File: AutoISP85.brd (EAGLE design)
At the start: 10.5 x 38.1 mm, 4 parts, among them J1 MCU, J2 BOARD, U1 ATTINY85, U2 BOARD

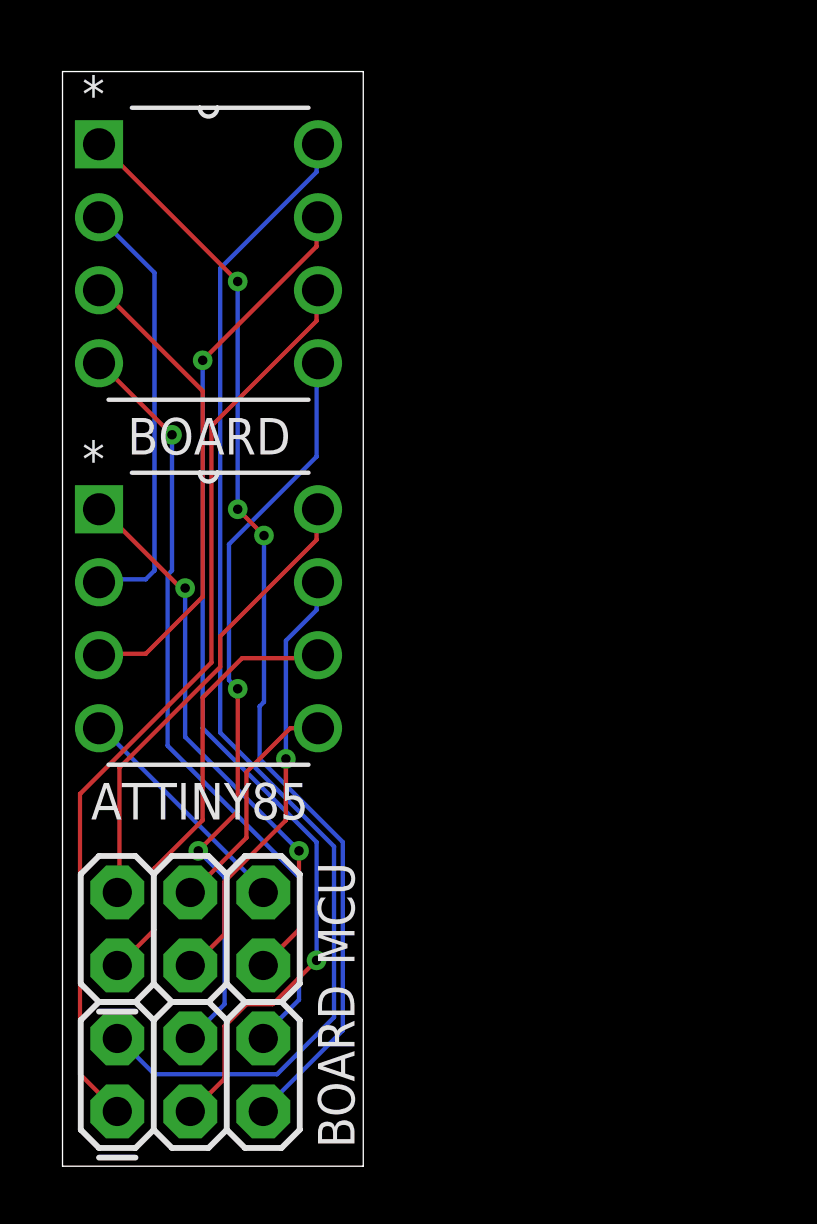
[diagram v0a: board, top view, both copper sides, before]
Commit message: Revise boards for better labelling and sane orientation, add AutoISP328
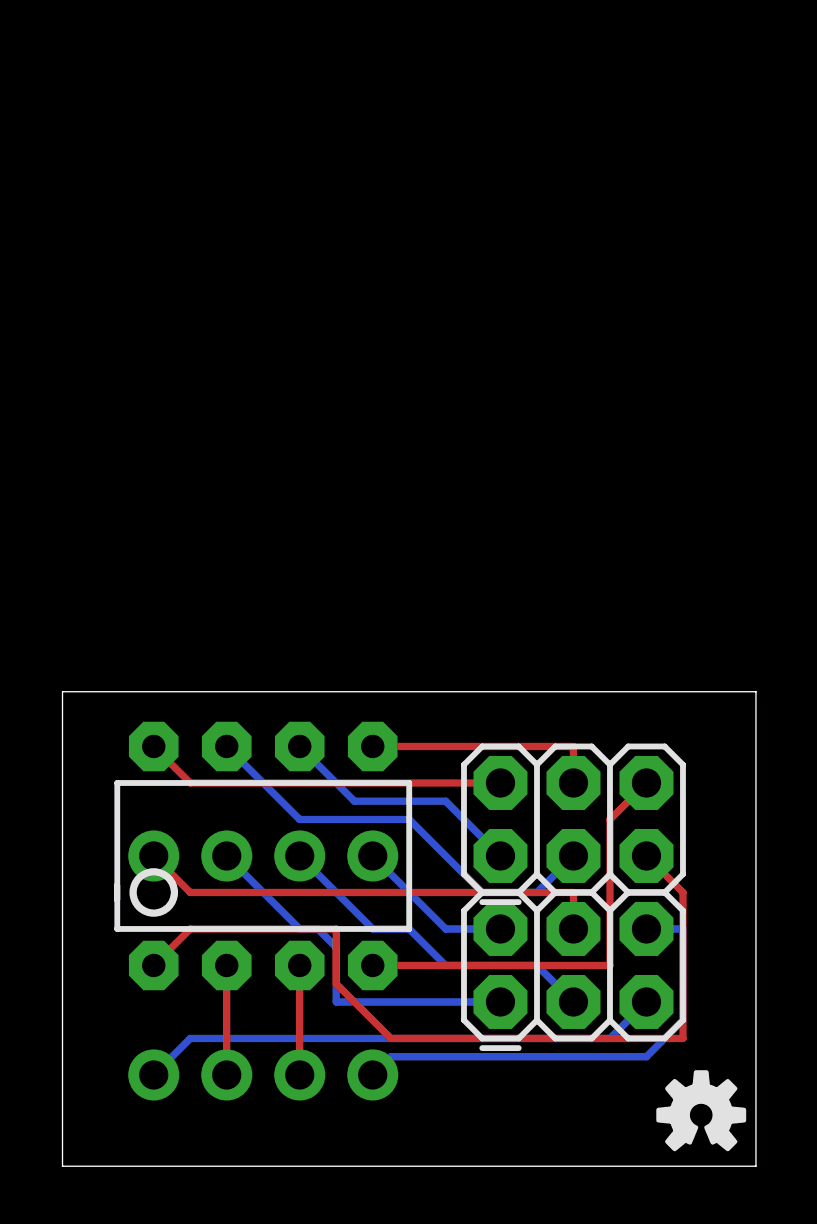
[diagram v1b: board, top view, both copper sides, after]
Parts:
- removed U2: BOARD, Atmel_By_element14_Batch_1-00:DIP254P762X533-8
- added CN1, CN3: 1X4-CLEANBIG, adafruit:1X04-CLEANBIG
- added U$1: (no value), SparkFun-Aesthetics:OSHW-LOGO-S
- U1: value ATTINY85 -> TINY85-20-DIP; device Atmel_By_element14_Batch_1-00:DIP254P762X533-8 -> SparkFun-DigitalIC:DIP08
- moved J1 13.9 mm to (15.2, 10.8)
- moved J2 13.9 mm to (15.2, 5.71)
- moved U1 4.84 mm to (6.99, 10.8)
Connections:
- removed net N$13: U1.2, U2.2
- removed net N$14: U1.3, U2.3
- new net N$5: CN1.1, J2.5
- new net N$6: CN1.2, U1.2
- net N$10: now also CN3.2, J2.1; no longer J2.4, U2.5
- net N$11: now also CN3.3, J2.3; no longer J2.1, U2.6
- net N$12: now also CN3.4, J2.2; no longer J2.3, U2.7
- net N$7: now also CN1.3, U1.3; no longer J2.5, U2.1
- net N$8: now also CN1.4, J2.6; no longer J2.2, U2.8
- net N$9: now also CN3.1, J2.4; no longer J2.6, U2.4
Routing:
- net N$7: track 38.5 -> 3.81 mm, vias 3 -> 0
- net N$12: track 36.8 -> 5.50 mm, vias 2 -> 0
- net N$8: track 42.3 -> 16.0 mm
- net N$11: track 32.6 -> 11.6 mm
- net N$5: track 0.00 -> 18.2 mm
- net N$14: track 16.7 -> 0.00 mm
- net N$13: track 15.2 -> 0.00 mm
- net N$10: track 26.3 -> 12.7 mm, vias 2 -> 0
- net N$9: track 27.0 -> 16.4 mm, vias 1 -> 0
- net N$1: track 19.4 -> 28.5 mm, vias 2 -> 0
- net N$3: track 8.16 -> 15.1 mm
- net N$15: track 15.2 -> 8.56 mm
- net N$6: track 0.00 -> 3.81 mm
- net N$2: track 16.3 -> 12.6 mm
- net N$16: track 15.2 -> 14.7 mm, vias 1 -> 0
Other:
- board size 10.5 x 38.1 mm -> 24.1 x 16.5 mm
- board text added: "*"
- board text added: "AutoISP85 v1.2"
- board text added: "µTh '15 CC BY"
- board text removed: "AutoISP85 v1.0 µTh 2014"

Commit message: AutoISP85 1.3 (Fix flipped pin header) Add BOM
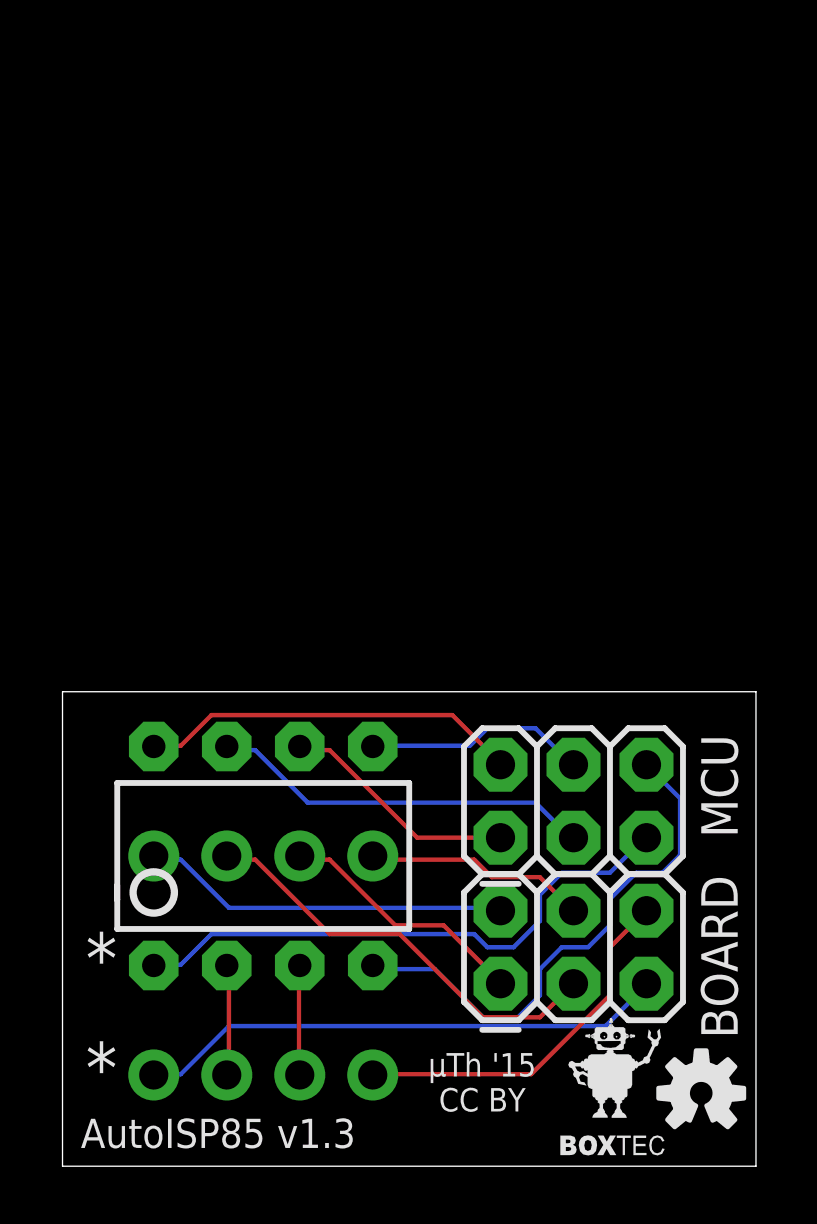
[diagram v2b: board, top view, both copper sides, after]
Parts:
- added U$2: (no value), SparkFun-Aesthetics:OSHW-LOGO-S
- U$1: device SparkFun-Aesthetics:OSHW-LOGO-S -> Boxtec-veclogo:ROBOXTEC-VECLOGO-MICRO
- moved U$1 3.47 mm to (19.1, 3.17)
- moved J1 0.63 mm to (15.2, 11.4)
- moved J2 0.63 mm to (15.2, 6.35)
- flipped CN3 to the bottom
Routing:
- net N$1: track 28.5 -> 19.9 mm
- net N$9: track 16.4 -> 7.83 mm
- net N$12: track 5.50 -> 13.0 mm
- net N$10: track 12.7 -> 8.86 mm
- net N$3: track 15.1 -> 18.5 mm
- net N$11: track 11.6 -> 14.9 mm
- net N$8: track 16.0 -> 12.9 mm
- net N$16: track 14.7 -> 13.4 mm
- net N$2: track 12.6 -> 13.3 mm
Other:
- board text added: "AutoISP85 v1.3"
- board text removed: "AutoISP85 v1.2"
